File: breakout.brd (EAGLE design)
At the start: 44.5 x 25.4 mm, 21 parts

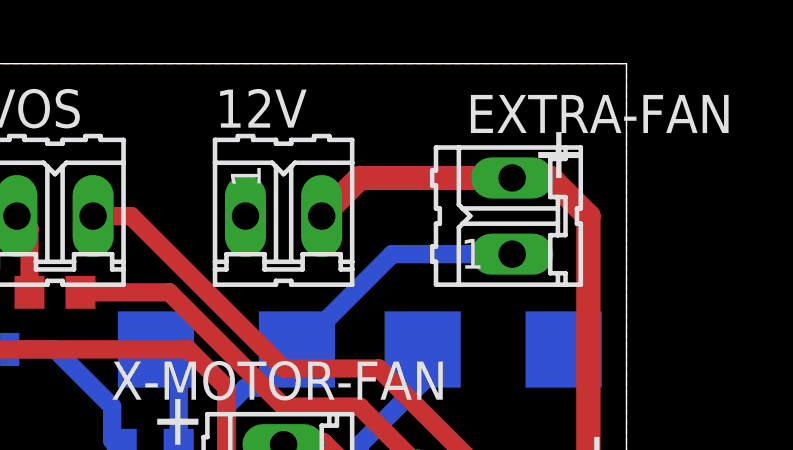
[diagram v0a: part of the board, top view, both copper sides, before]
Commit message: Adjusting labels and positioning.
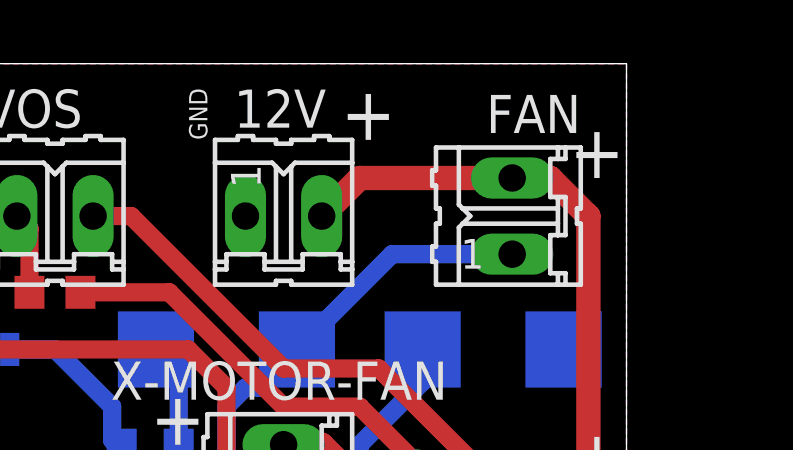
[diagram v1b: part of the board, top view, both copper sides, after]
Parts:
- renumbered EXTRA-FAN to FAN
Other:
- board text added: "GND"
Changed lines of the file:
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@@
 <text x="33.655" y="5.08" size="1.778" layer="25">+</text>
 <text x="33.655" y="12.7" size="1.778" layer="25">+</text>
-<text x="46.355" y="21.59" size="1.778" layer="25">+</text>
+<text x="47.625" y="21.59" size="1.778" layer="25">+</text>
 <text x="47.625" y="11.43" size="1.778" layer="25">+</text>
 <text x="21.59" y="17.78" size="1.778" layer="25">4</text>
+<text x="40.005" y="22.86" size="1.778" layer="25">+</text>
+<text x="35.56" y="22.86" size="0.6096" layer="25" rot="R90">GND</text>
 </plain>
 <attributes>
@@
 <attribute name="VALUE" x="38.735" y="13.589" size="0.4064" layer="28" font="vector" rot="MR0"/>
 </element>
-<element name="EXTRA-FAN" library="con-amp-quick" package="02P" value="" x="45.72" y="20.32" smashed="yes" rot="R90">
+<element name="FAN" library="con-amp-quick" package="02P" value="" x="45.72" y="20.32" smashed="yes" rot="R90">
 <attribute name="MF" value="" x="45.72" y="20.32" size="1.778" layer="27" rot="R90" display="off"/>
 <attribute name="MPN" value="" x="45.72" y="20.32" size="1.778" layer="27" rot="R90" display="off"/>
-<attribute name="NAME" x="53.086" y="24.3586" size="1.27" layer="25" ratio="10" rot="R180"/>
+<attribute name="NAME" x="48.006" y="24.3586" size="1.27" layer="25" ratio="10" rot="R180"/>
 <attribute name="OC_FARNELL" value="unknown" x="45.72" y="20.32" size="1.778" layer="27" rot="R90" display="off"/>
 <attribute name="OC_NEWARK" value="unknown" x="45.72" y="20.32" size="1.778" layer="27" rot="R90" display="off"/>
@@
 <attribute name="VALUE" x="41.9354" y="9.144" size="1.27" layer="27" ratio="10" rot="R90"/>
 </element>
-<element name="12V" library="con-amp-quick" package="02P" value="" x="38.1" y="20.32">
+<element name="12V" library="con-amp-quick" package="02P" value="" x="38.1" y="20.32" smashed="yes">
 <attribute name="MF" value="" x="38.1" y="20.32" size="1.778" layer="27" display="off"/>
 <attribute name="MPN" value="" x="38.1" y="20.32" size="1.778" layer="27" display="off"/>
+<attribute name="NAME" x="36.449" y="23.2664" size="1.27" layer="25" ratio="10"/>
 <attribute name="OC_FARNELL" value="unknown" x="38.1" y="20.32" size="1.778" layer="27" display="off"/>
 <attribute name="OC_NEWARK" value="unknown" x="38.1" y="20.32" size="1.778" layer="27" display="off"/>
+<attribute name="VALUE" x="35.814" y="16.4846" size="1.27" layer="27" ratio="10"/>
 </element>
 <element name="U$1" library="headers(2mm)" package="1X6" value="1X6" x="25.4" y="2.54"/>
@@
 <contactref element="RADIATOR-FAN" pad="2"/>
 <contactref element="X-MOTOR-FAN" pad="2"/>
-<contactref element="EXTRA-FAN" pad="2"/>
+<contactref element="FAN" pad="2"/>
 <wire x1="48.26" y1="7.62" x2="48.26" y2="20.32" width="0.8128" layer="1"/>
 <wire x1="48.26" y1="7.62" x2="46.99" y2="6.35" width="0.8128" layer="1"/>
@@
 <signal name="N$13">
 <contactref element="D3" pad="C"/>
-<contactref element="EXTRA-FAN" pad="1"/>
+<contactref element="FAN" pad="1"/>
 <contactref element="T3" pad="C"/>
 <wire x1="33.655" y1="10.33" x2="34.46" y2="10.33" width="0.6096" layer="16"/>
